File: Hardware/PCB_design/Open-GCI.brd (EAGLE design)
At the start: 100 x 94 mm, 29 parts, among them IC1 IC1, IC2 IC2, X1 USB

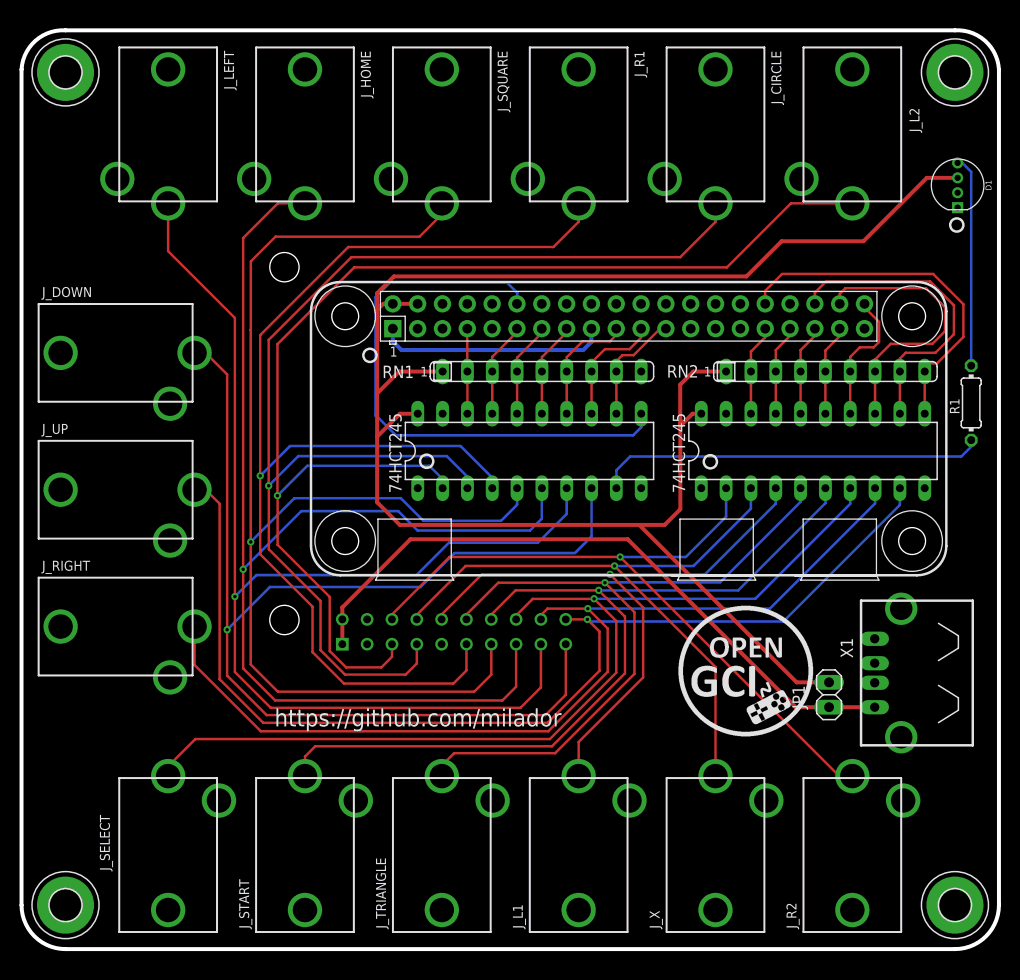
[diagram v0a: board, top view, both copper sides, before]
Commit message: Updated PCB, Component listand gerber files
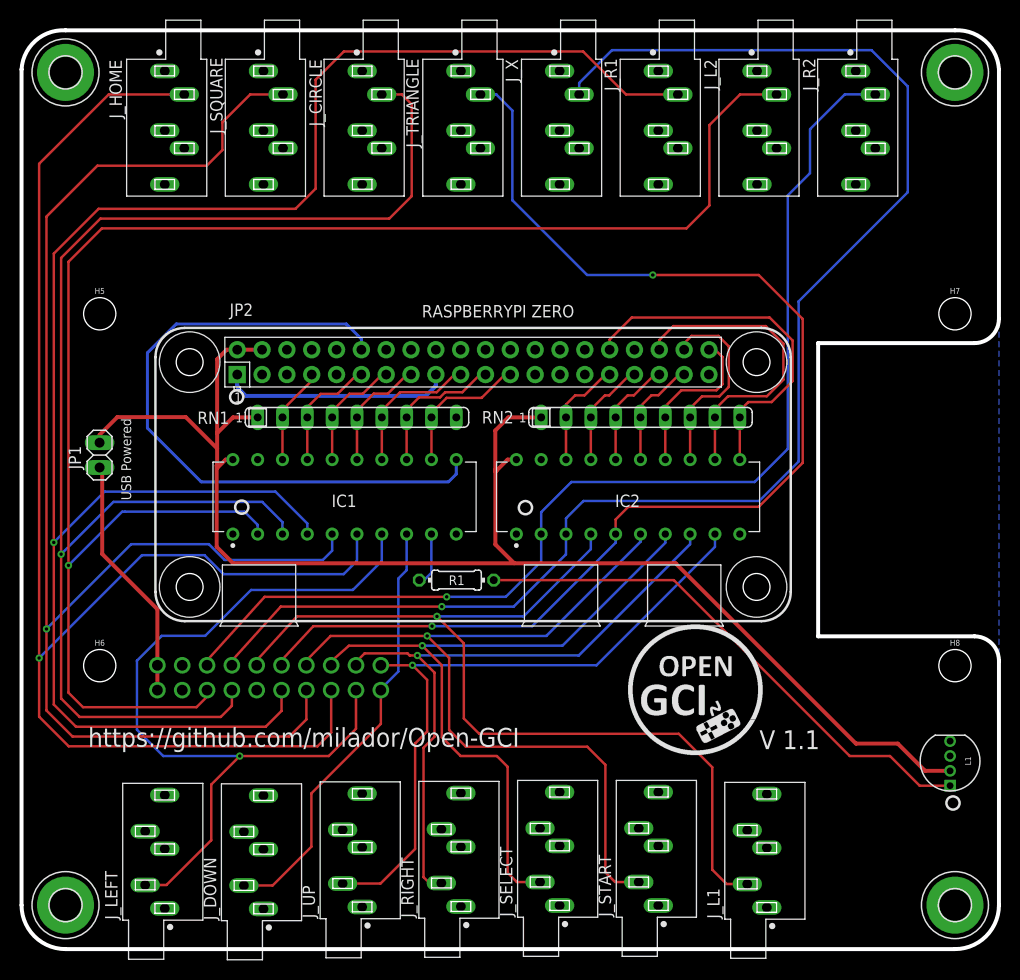
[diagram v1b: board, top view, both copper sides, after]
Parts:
- removed D1: RGB LED, open-gci-package:NEOPIXEL-RGB-THRU
- removed U$1: RPI-ZERO, open-gci-package:RASPBERRYPI_BASTELSTUBE_V13_RASPI_BOARD_B+_FULL
- removed U$2: BROOK, open-gci-package:BROOK
- removed X1: USB, open-gci-package:PN87520-S
- added H5, H6, H7, H8: (no value), SparkFun-Hardware:STAND-OFF
- added JP2: RASPBERRYPI ZERO, milador:RASPBERRYPI_ZERO
- added JP3: BROOK, milador:CONN_2X10
- added L1: NEOPIXELS, milador:NEOPIXELS-5MM
- IC1: value IC1 -> SN74HCT245; device open-gci-package:74HCT245 -> milador:SN74HCT245
- IC2: value IC2 -> SN74HCT245; device open-gci-package:74HCT245 -> milador:SN74HCT245
- J_CIRCLE, J_DOWN, J_HOME, J_L1, J_L2, J_LEFT, J_R1, J_R2, J_RIGHT, J_SELECT, J_SQUARE, J_START, J_TRIANGLE, J_UP, J_X: value MJ-3536N -> SJ1-3535NG; device con-cuistack:MJ-3536N -> milador:CUI_SJ1-3535NG
- R1: device rcl:0204/7 -> milador:0204/7
- RN1, RN2: device resistor-sil:SIL9 -> milador:SIL9
- moved J_X 87.3 mm to (55.0, 89.8), turned to 270 degrees
- moved J_TRIANGLE 85.9 mm to (45.0, 89.8), turned to 270 degrees
- moved J_LEFT 85.8 mm to (14.7, 4.16), turned to 90 degrees
- moved J_R2 85.8 mm to (85.3, 89.8), turned to 270 degrees
- moved JP1 78.6 mm to (7.99, 50.5)
- moved J_DOWN 60.6 mm to (24.8, 4.11), turned to 90 degrees
- moved R1 55.7 mm to (44.5, 37.8), turned to 180 degrees
- moved J_UP 52.7 mm to (34.9, 4.31), turned to 90 degrees
- moved J_RIGHT 50.0 mm to (45.0, 4.36), turned to 90 degrees
- moved J_SELECT 40.1 mm to (55.0, 4.46), turned to 90 degrees
- moved J_START 36.2 mm to (65.2, 4.46), turned to 90 degrees
- moved J_CIRCLE 36.2 mm to (34.9, 89.8), turned to 270 degrees
- moved IC1 19.5 mm to (33.0, 46.3), turned to 90 degrees
- moved IC2 19.5 mm to (62.1, 46.3), turned to 90 degrees
- moved RN1 19.5 mm to (34.3, 54.4)
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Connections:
- removed net N$1: IC1.A0, J_L2.2, U$2.L2
- removed net N$10: IC2.A2, J_L1.2, U$2.L1
- removed net N$11: IC2.A3, J_TRIANGLE.2, U$2.TRIANGLE
- removed net N$12: IC2.A4, J_START.2, U$2.START
- removed net N$13: IC2.A5, J_SELECT.2, U$2.SELECT
- removed net N$14: IC2.A6, J_RIGHT.2, U$2.RIGHT
- removed net N$15: IC2.A7, J_UP.2, U$2.UP
- removed net N$16: IC1.B0, RN1.2, U$1.7
- removed net N$17: IC1.B1, RN1.3, U$1.11
- removed net N$18: IC1.B2, RN1.4, U$1.13
- removed net N$19: IC1.B3, RN1.5, U$1.15
- removed net N$2: IC1.A1, J_CIRCLE.2, U$2.CIRCLE
- removed net N$20: IC1.B5, RN1.7, U$1.21
- removed net N$21: IC1.B4, RN1.6, U$1.19
- removed net N$22: IC1.B6, RN1.8, U$1.23
- removed net N$23: IC1.B7, U$1.12
- removed net N$24: IC2.B1, RN2.3, U$1.33
- removed net N$25: IC2.B0, RN2.2, U$1.31
- removed net N$26: IC2.B2, RN2.4, U$1.35
- removed net N$27: IC2.B3, RN2.5, U$1.37
- removed net N$28: IC2.B4, RN2.6, U$1.40
- removed net N$29: IC2.B5, RN2.7, U$1.38
- removed net N$3: IC1.A2, J_R1.2, U$2.R1
- removed net N$30: IC2.B6, RN2.8, U$1.36
- removed net N$31: IC2.B7, RN2.9, U$1.32
- removed net N$4: IC1.A3, J_SQUARE.2, U$2.SQUARE
- removed net N$5: IC1.A4, J_HOME.2, U$2.HOME
- removed net N$6: IC1.A5, J_LEFT.2, U$2.LEFT
- removed net N$7: IC1.A6, J_DOWN.2, U$2.DOWN
- removed net N$8: IC2.A0, J_R2.2, U$2.R2
- removed net N$9: IC2.A1, J_X.2, U$2.X
- new net NGP11: IC1.17, JP2.11, RN1.3
- new net NGP12: IC1.11, JP2.12
- new net NGP13: IC1.16, JP2.13, RN1.4
- new net NGP15: IC1.15, JP2.15, RN1.5
- new net NGP19: IC1.14, JP2.19, RN1.6
- new net NGP21: IC1.13, JP2.21, RN1.7
- new net NGP23: IC1.12, JP2.23, RN1.8
- new net NGP31: IC2.18, JP2.31, RN2.2
- new net NGP32: IC2.11, JP2.32, RN2.9
- new net NGP33: IC2.17, JP2.33, RN2.3
- new net NGP35: IC2.16, JP2.35, RN2.4
- new net NGP36: IC2.12, JP2.36, RN2.8
- new net NGP37: IC2.15, JP2.37, RN2.5
- new net NGP38: IC2.13, JP2.38, RN2.7
- new net NGP40: IC2.14, JP2.40, RN2.6
- new net NGP7: IC1.18, JP2.7, RN1.2
- new net NJ_CIR: IC1.3, JP3.CIRCLE, J_CIRCLE.2
- new net NJ_DOWN: IC1.8, JP3.DOWN, J_DOWN.2
- new net NJ_HOME: IC1.6, JP3.HOME, J_HOME.2
- new net NJ_L1: IC2.4, JP3.L1, J_L1.2
- new net NJ_L2: IC1.2, JP3.L2, J_L2.2
- new net NJ_LEFT: IC1.7, JP3.LEFT, J_LEFT.2
- new net NJ_R1: IC1.4, JP3.R1, J_R1.2
- new net NJ_R2: IC2.2, JP3.R2, J_R2.2
- new net NJ_RIGHT: IC2.8, JP3.RIGHT, J_RIGHT.2
- new net NJ_SELECT: IC2.7, JP3.SELECT, J_SELECT.2
- new net NJ_SQU: IC1.5, JP3.SQUARE, J_SQUARE.2
- new net NJ_START: IC2.6, JP3.START, J_START.2
- new net NJ_TRI: IC2.5, JP3.TRIANGLE, J_TRIANGLE.2
- new net NJ_UP: IC2.9, JP3.UP, J_UP.2
- new net NJ_X: IC2.3, JP3.X, J_X.2
- net +3V3: now also JP2.1, JP2.17; no longer U$1.1, U$1.17
- net +5V: now also IC1.20, IC2.20, JP2.2, JP2.4, L1.2; no longer D1.3, IC1.VCC, IC2.VCC, U$1.2, U$1.4
- net +5V/2: now also JP3.VCC1, JP3.VCC2; no longer U$2.VCC1, U$2.VCC2, X1.1
- net GND: now also IC1.1, IC1.10, IC1.19, IC2.1, IC2.10, IC2.19, JP2.14, JP2.20, JP2.25, JP2.30, JP2.34, JP2.39, JP2.6, JP2.9, JP3.GND1, JP3.GND2, JP3.GND3, L1.3, L1.4; no longer D1.1, D1.2, IC1.DIR, IC1.GND, IC1.OE, IC2.DIR, IC2.GND, IC2.OE, U$1.14, U$1.20, U$1.25, U$1.30, U$1.34, U$1.39, U$1.6, U$1.9, U$2.GND1, U$2.GND2, U$2.GND3, X1.2, X1.3, X1.4, X1.S1, X1.S2
- net N$32: now also IC1.9; no longer IC1.A7
- net N$33: now also L1.1; no longer D1.4
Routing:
- net NJ_R1: track 0.00 -> 184.5 mm, vias 0 -> 1
- net NJ_L2: track 0.00 -> 167.5 mm, vias 0 -> 1
- net NJ_HOME: track 0.00 -> 151.4 mm, vias 0 -> 1
- net NJ_X: track 0.00 -> 149.9 mm, vias 0 -> 1
- net NJ_SQU: track 0.00 -> 148.6 mm, vias 0 -> 1
- net NJ_CIR: track 0.00 -> 143.7 mm, vias 0 -> 1
- net N$6: track 129.0 -> 0.00 mm, vias 1 -> 0
- net N$1: track 126.9 -> 0.00 mm, vias 1 -> 0
- net NJ_TRI: track 0.00 -> 126.3 mm, vias 0 -> 2
- net N$4: track 126.0 -> 0.00 mm, vias 1 -> 0
- net N$7: track 123.6 -> 0.00 mm, vias 1 -> 0
- net N$2: track 123.6 -> 0.00 mm, vias 1 -> 0
- net N$5: track 123.5 -> 0.00 mm, vias 1 -> 0
- net N$3: track 121.7 -> 0.00 mm, vias 1 -> 0
- net NJ_R2: track 0.00 -> 113.8 mm, vias 0 -> 1
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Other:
- outline, holes or cut-outs redrawn
- board text added: "USB Powered"
- board text added: "V 1.1"
- board text added: "https://github.com/milador/Open-GCI"
- board text removed: "https://github.com/milador"
